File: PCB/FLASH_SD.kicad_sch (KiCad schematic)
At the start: 31 parts, among them J501 MEM2090-00-145-00-A_REVA, U501 EMMC04G-W627-M06U, U502 HSP051-4M10, U503 HSP051-4M10

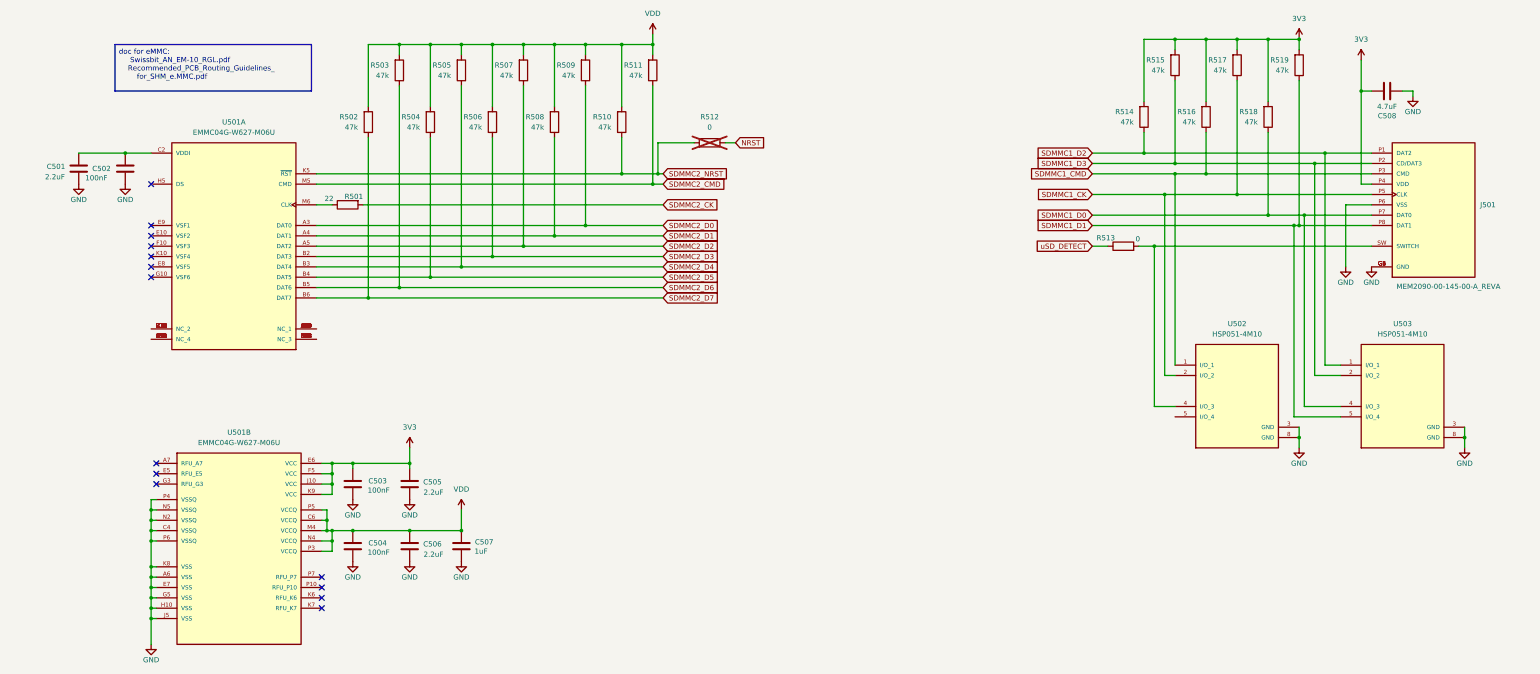
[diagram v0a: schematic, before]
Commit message: PCD_UPDATE
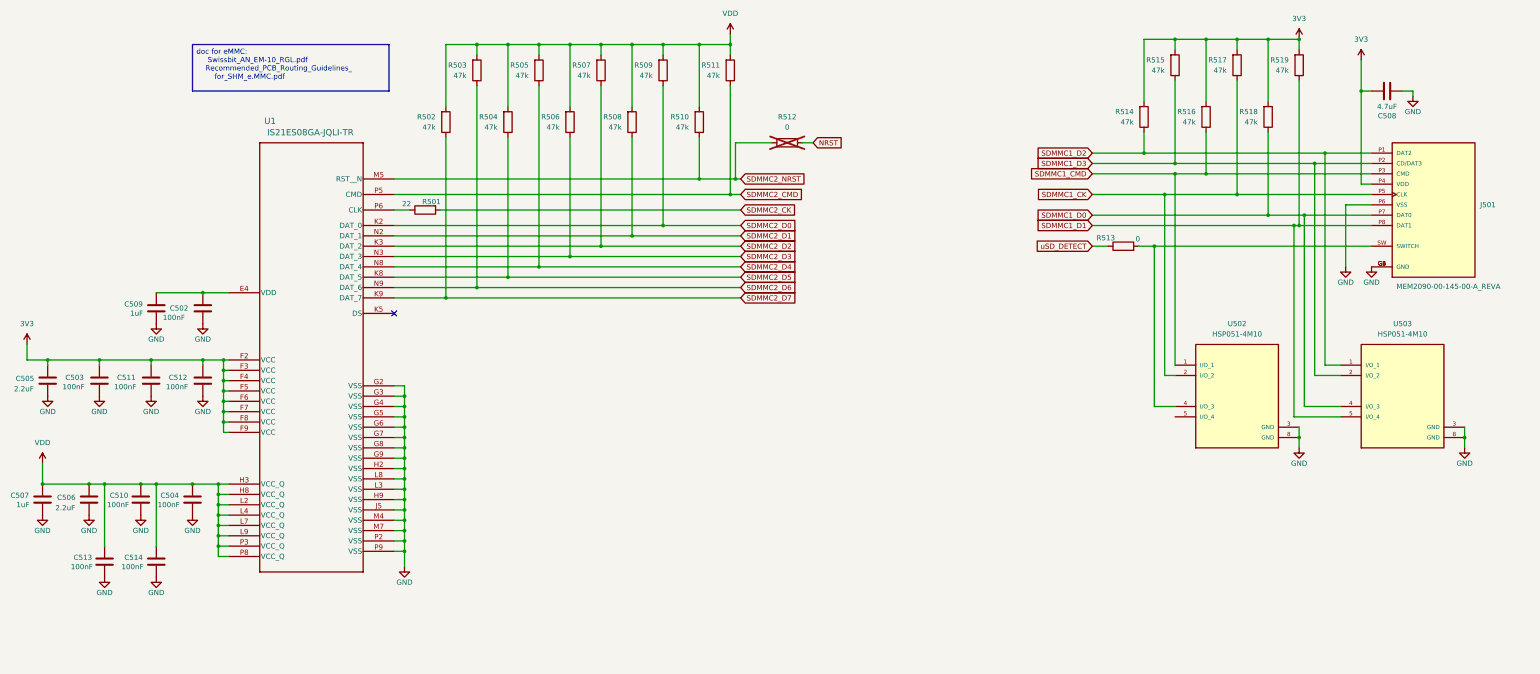
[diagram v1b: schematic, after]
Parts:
- removed C501: 2.2uF, Capacitor_SMD:C_0402_1005Metric, symbol Device:C
- removed U501: EMMC04G-W627-M06U, lib:BGA153N50P14X14_1300X1150X100N, symbol EMMC04G-W627-M06U:EMMC04G-W627-M06U
- added C509: 1uF, Capacitor_SMD:C_0402_1005Metric, symbol Device:C
- added C510, C511, C512, C513, C514: 100nF, Capacitor_SMD:C_0402_1005Metric, symbol Device:C
- added U1: IS21ES08GA-JQLI-TR, FBGA100_ISI, symbol IS21ES08GA-JQLI:IS21ES08GA-JQLI-TR
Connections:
- net 3V3: now also C511.2, C512.2, U1.F2 (VCC), U1.F3 (VCC), U1.F4 (VCC), U1.F5 (VCC), U1.F6 (VCC), U1.F7 (VCC), U1.F8 (VCC), U1.F9 (VCC)
- net GND: now also C509.2, C510.1, C511.1, C512.1, C513.1, C514.1, U1.G2 (VSS), U1.G3 (VSS), U1.G4 (VSS), U1.G5 (VSS), U1.G6 (VSS), U1.G7 (VSS), U1.G8 (VSS), U1.G9 (VSS), U1.H2 (VSS), U1.H9 (VSS), U1.J5 (VSS), U1.L3 (VSS), U1.L8 (VSS), U1.M4 (VSS), U1.M7 (VSS), U1.P2 (VSS), U1.P9 (VSS)
- net SDMMC2_CMD: now also U1.P5 (CMD)
- net SDMMC2_D0: now also U1.K2 (DAT_0)
- net SDMMC2_D1: now also U1.N2 (DAT_1)
- net SDMMC2_D2: now also U1.K3 (DAT_2)
- net SDMMC2_D3: now also U1.N3 (DAT_3)
- net SDMMC2_D4: now also U1.N8 (DAT_4)
- net SDMMC2_D5: now also U1.K8 (DAT_5)
- net SDMMC2_D6: now also U1.N9 (DAT_6)
- net SDMMC2_D7: now also U1.K9 (DAT_7)
- net SDMMC2_NRST: now also U1.M5 (RST__N)
- net VDD: now also C510.2, C513.2, C514.2, U1.H3 (VCC_Q), U1.H8 (VCC_Q), U1.L2 (VCC_Q), U1.L4 (VCC_Q), U1.L7 (VCC_Q), U1.L9 (VCC_Q), U1.P3 (VCC_Q), U1.P8 (VCC_Q)
- net at C502.2: now also C509.1, U1.E4 (VDD)
- net at R501.1: now also U1.P6 (CLK)
- no-connect marks 14 -> 1
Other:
- moved on the sheet: C502, C503, C504, C505, C506, C507, R501, R502, R503, R504, R505, R506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
